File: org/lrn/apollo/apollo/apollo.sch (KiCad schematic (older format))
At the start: 2 parts, among them U1 74HC595, U2 5461AS-1

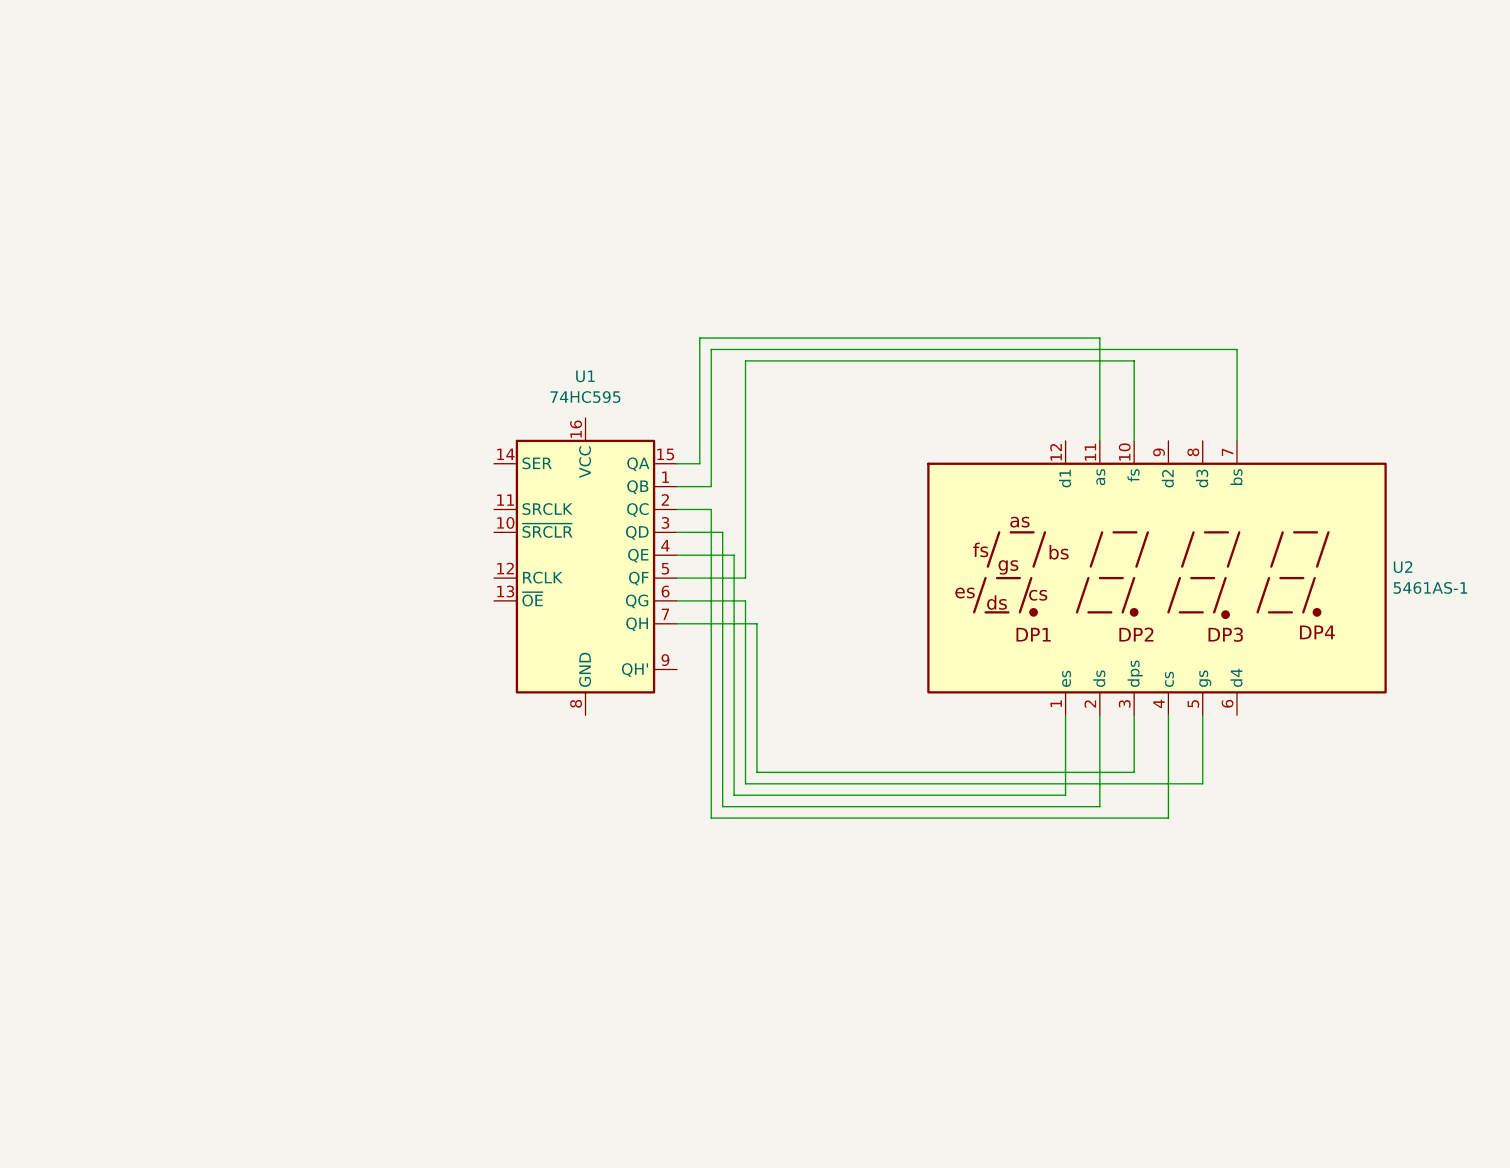
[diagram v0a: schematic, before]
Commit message: apollo pcb
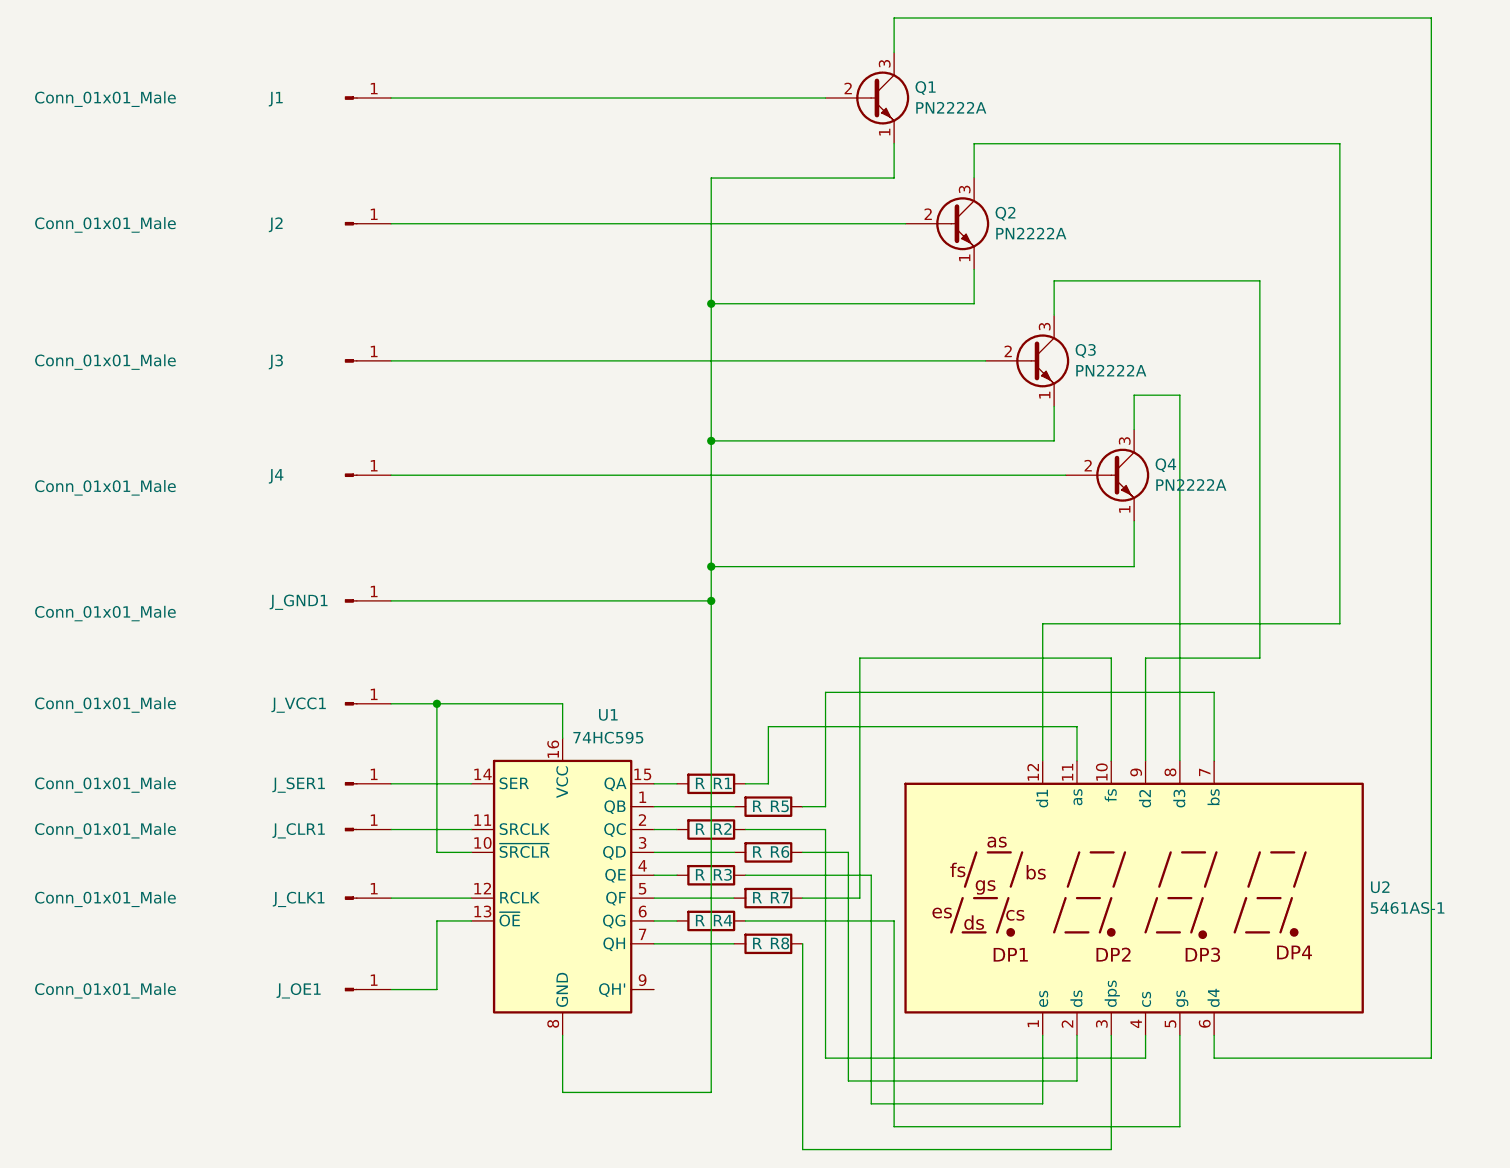
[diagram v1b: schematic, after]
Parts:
- added J1, J2, J3, J4, J_CLK1, J_CLR1, J_GND1, J_OE1, J_SER1, J_VCC1: Conn_01x01_Male, Connector_Pin:Pin_D0.7mm_L6.5mm_W1.8mm_FlatFork, symbol Connector:Conn_01x01_Male
- added Q1, Q2, Q3, Q4: PN2222A, Package_TO_SOT_THT:TO-92_Inline, symbol Transistor_BJT:PN2222A
- added R1, R2, R3, R4, R5, R6, R7, R8: R, Resistor_THT:R_Axial_DIN0204_L3.6mm_D1.6mm_P5.08mm_Horizontal, symbol Device:R
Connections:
- net at U2.1 (es): now also R3.1; no longer U1.4 (QE)
- net at U2.10 (fs): now also R7.1; no longer U1.5 (QF)
- net at U2.11 (as): now also R1.1; no longer U1.15 (QA)
- net at U2.12 (d1): now also Q2.3 (C)
- net at U2.2 (ds): now also R6.1; no longer U1.3 (QD)
- net at U2.3 (dps): now also R8.1; no longer U1.7 (QH)
- net at U2.4 (cs): now also R2.1; no longer U1.2 (QC)
- net at U2.5 (gs): now also R4.1; no longer U1.6 (QG)
- net at U2.6 (d4): now also Q1.3 (C)
- net at U2.7 (bs): now also R5.1; no longer U1.1 (QB)
- net at U2.8 (d3): now also Q4.3 (C)
- net at U2.9 (d2): now also Q3.3 (C)
- net at U1.10 (~SRCLR): now also U1.16 (VCC), J_VCC1.1 (Pin_1)
- net at U1.11 (SRCLK): now also J_CLR1.1 (Pin_1)
- net at U1.12 (RCLK): now also J_CLK1.1 (Pin_1)
- net at U1.13 (~OE): now also J_OE1.1 (Pin_1)
- net at U1.14 (SER): now also J_SER1.1 (Pin_1)
- net at U1.8 (GND): now also J_GND1.1 (Pin_1), Q1.1 (E), Q2.1 (E), Q3.1 (E), Q4.1 (E)
- new net: R5.2, U1.1 (QB)
- new net: R1.2, U1.15 (QA)
- new net: R2.2, U1.2 (QC)
- new net: R6.2, U1.3 (QD)
- new net: R3.2, U1.4 (QE)
- new net: R7.2, U1.5 (QF)
- new net: R4.2, U1.6 (QG)
- new net: R8.2, U1.7 (QH)
- new net: J2.1 (Pin_1), Q2.2 (B)
- new net: J3.1 (Pin_1), Q3.2 (B)
- new net: J4.1 (Pin_1), Q4.2 (B)
- new net: J1.1 (Pin_1), Q1.2 (B)
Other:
- moved on the sheet: U1, U2
